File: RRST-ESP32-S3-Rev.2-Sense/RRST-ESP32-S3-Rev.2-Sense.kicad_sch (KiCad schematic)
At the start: 69 parts, among them J1 Conn_01x22_Pin, J10 Conn_01x02_Socket, J11 Conn_01x02_Socket, J12 Conn_01x02_Socket, J2 USB_C_Receptacle_USB2.0_16P, J3 Conn_01x22_Pin, J4 Conn_01x04_Socket, J5 Conn_01x04_Socket, J6 Conn_01x04_Socket, J7 Conn_01x04_Socket, J8 Conn_01x04_Socket, J9 Conn_01x02_Socket, SW1 SW_Push, SW2 SW_Push, U1 ESP32-S3-WROOM-1, U2 LD1117S33TR_SOT223, U4 MCP2561-E-SN

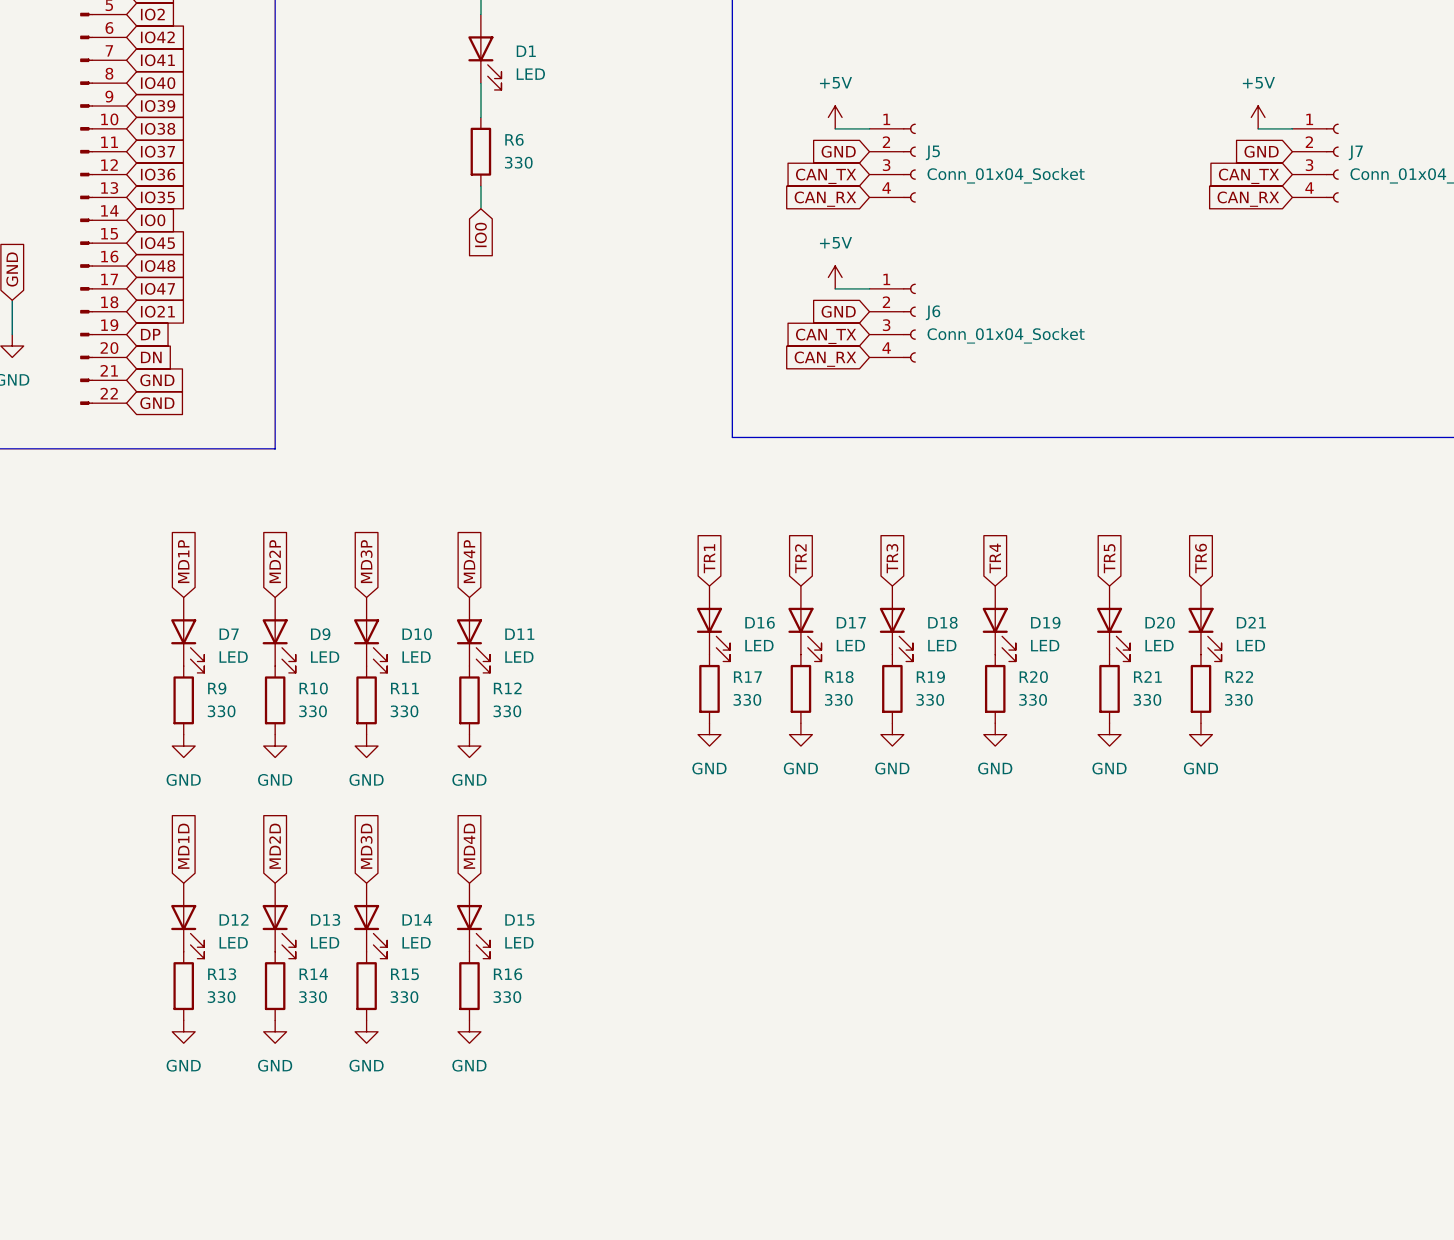
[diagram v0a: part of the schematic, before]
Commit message: 仮配置
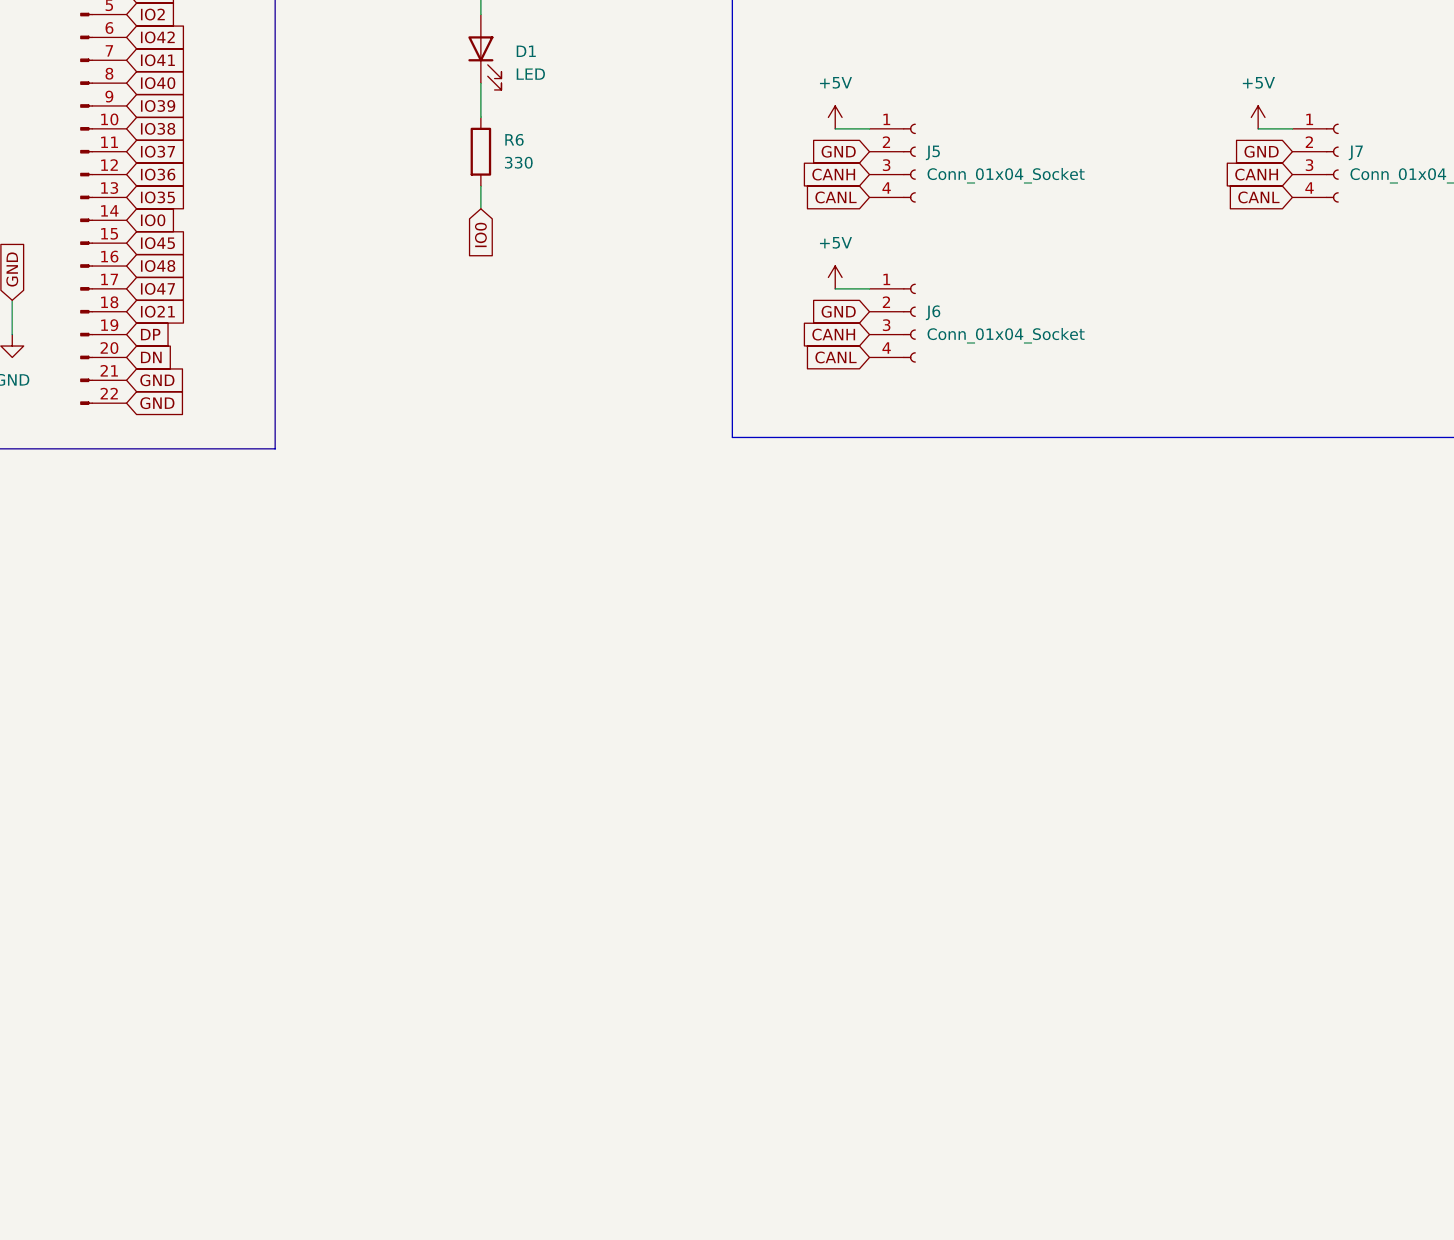
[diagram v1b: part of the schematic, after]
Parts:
- removed D10, D11, D12, D13, D14, D15, D16, D17, D18, D19, D20, D21, D7, D9: LED, LED_SMD:LED_0603_1608Metric, symbol Device:LED
- removed R10, R11, R12, R13, R14, R15, R16, R17, R18, R19, R20, R21, R22, R9: 330, Resistor_SMD:R_0603_1608Metric, symbol Device:R
- J10, J11, J12, J9: footprint Connector_JST:JST_XH_S2B-XH-A-1_1x02_P2.50mm_Horizontal -> Connector_JST:JST_XH_B2B-XH-A_1x02_P2.50mm_Vertical
- J4, J8: footprint Connector_JST:JST_XH_S4B-XH-A-1_1x04_P2.50mm_Horizontal -> Connector_JST:JST_XH_B4B-XH-A_1x04_P2.50mm_Vertical
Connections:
- net CANH: now also J5.3 (Pin_3), J6.3 (Pin_3), J7.3 (Pin_3)
- net CANL: now also J5.4 (Pin_4), J6.4 (Pin_4), J7.4 (Pin_4)
- net CAN_RX: no longer J5.4 (Pin_4), J6.4 (Pin_4), J7.4 (Pin_4)
- net CAN_TX: no longer J5.3 (Pin_3), J6.3 (Pin_3), J7.3 (Pin_3)
